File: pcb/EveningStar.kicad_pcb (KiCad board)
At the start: 2 copper layers, 107 x 97.2 mm, 153 parts, among them J2 DEBUG, P1 WJ15EDGRC-3.81-2P, Q1 2N7002, U1 78L05G, U11 15uH, U3 ISO6721RBDR, U5 74HC14D, U6 LMR38020SDDAR, U7 ESP32-C6-WROOM-1-N8, U8 GD5F2GM7UEYIGR, U9 W5500, X1 32.768kHz, Y1 25MHz

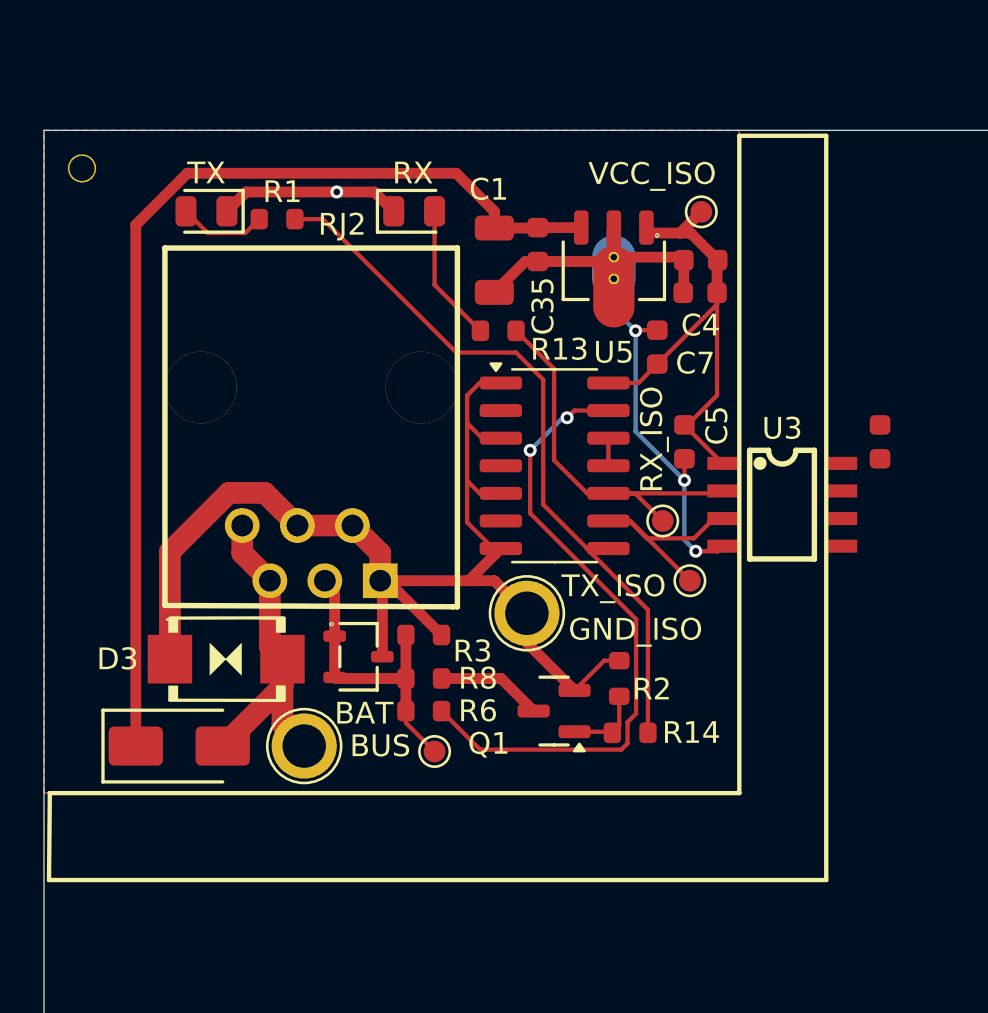
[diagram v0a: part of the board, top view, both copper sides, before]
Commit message: pcb(mb_frontend): optimise layout
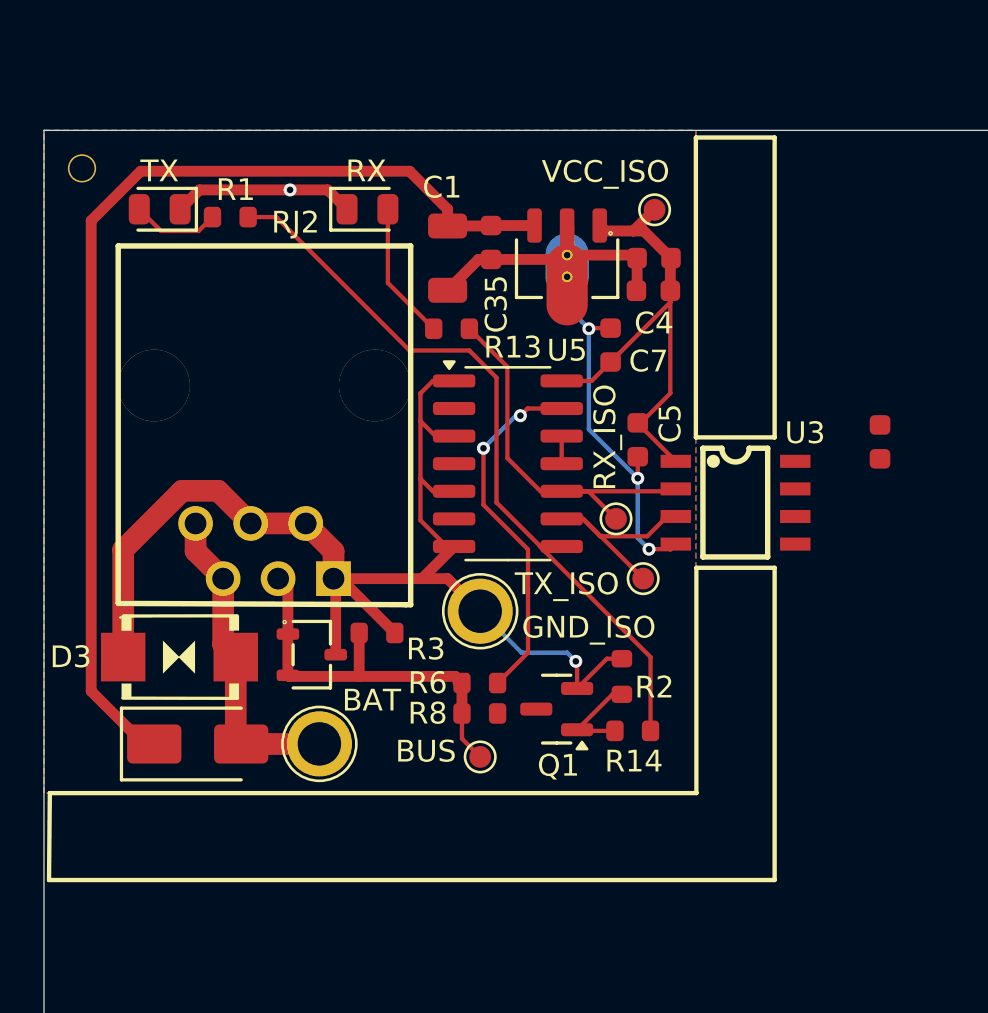
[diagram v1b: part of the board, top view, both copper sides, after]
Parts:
- moved R8 3.04 mm to (58.4, 72.5)
- moved R6 2.88 mm to (58.4, 71.1)
- moved TP21 2.15 mm to (66.5, 49.3)
- moved C1 2.15 mm to (57.0, 51.5)
- moved C35 2.15 mm to (59.0, 50.8)
- moved D3 2.15 mm to (44.6, 69.9)
- moved D4 2.15 mm to (43.7, 49.3)
- moved D6 2.15 mm to (53.3, 49.3)
- moved D7 2.15 mm to (50.7, 69.8)
- moved R1 2.15 mm to (47.0, 49.7)
- moved R13 2.15 mm to (57.1, 54.8)
- moved R3 2.15 mm to (53.7, 68.8)
- moved RJ2 2.15 mm to (48.5, 65.0)
- moved TP25 2.15 mm to (58.5, 67.8)
- moved U5 2.15 mm to (59.7, 61.0)
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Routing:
- net Net-(R6-Pad2): track 29.4 -> 16.6 mm
- net /meterbus_frontend/BUS_ISO: track 13.8 -> 19.0 mm
- net Net-(Q1-D): track 4.86 -> 0.00 mm
- net GND_ISO: track 94.0 -> 96.2 mm, vias 4 -> 5
- net MB_PWR_ISO: track 16.5 -> 14.6 mm
- net Net-(U1-VIN): track 47.0 -> 48.4 mm
- net Net-(Q1-G): track 3.57 -> 4.57 mm
- net Net-(R1-Pad1): track 34.7 -> 35.7 mm
